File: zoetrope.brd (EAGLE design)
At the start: 68.6 x 53.3 mm, 9 parts

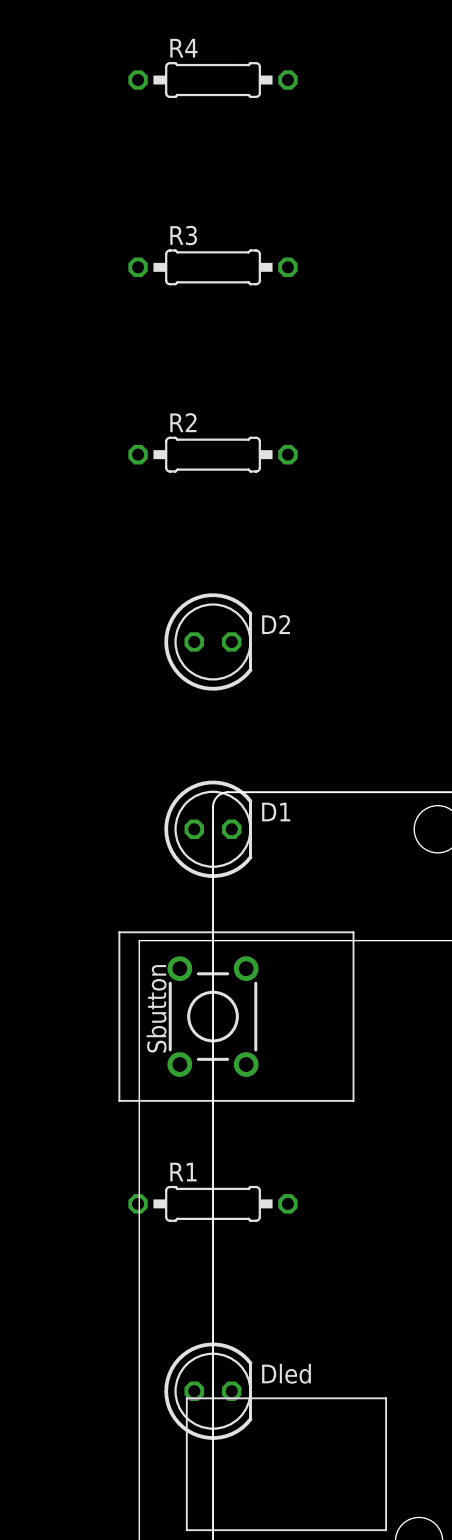
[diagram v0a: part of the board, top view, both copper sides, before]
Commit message: Added code and brd
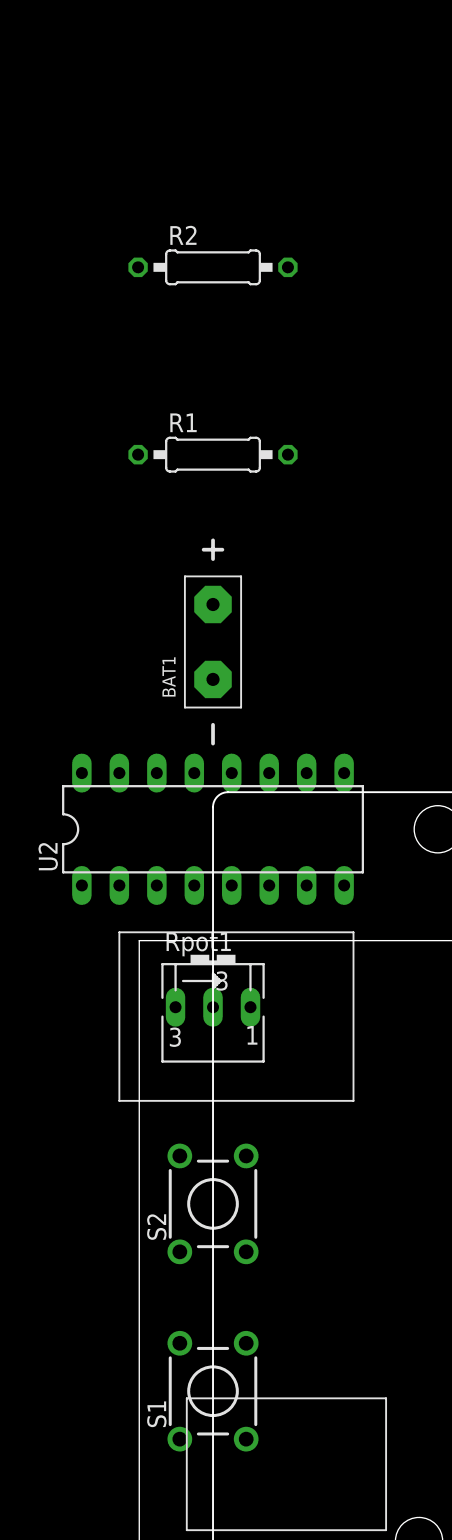
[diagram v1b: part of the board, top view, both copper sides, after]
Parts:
- removed D1, D2, Dled: (no value), AUTODESK_CIRCUITS_BREADBOARD:LED5MM
- removed R3, R4: 1k‎Ω, AUTODESK_CIRCUITS_BREADBOARD:0207/10
- removed Sbutton: (no value), AUTODESK_CIRCUITS_BREADBOARD:TL1105
- added BAT1: (no value), AUTODESK_CIRCUITS_BREADBOARD:DC-POWER
- added Rpot1: 250k‎Ω, AUTODESK_CIRCUITS_BREADBOARD:B25V
- added S1, S2: (no value), AUTODESK_CIRCUITS_BREADBOARD:TL1105
- added U2: (no value), AUTODESK_CIRCUITS_BREADBOARD:DIL16
- R1, R2: value 1k‎Ω -> 10000‎Ω
- moved R1 50.8 mm to (5.00, 86.3)
- moved R2 12.7 mm to (5.00, 99.0)
- renumbered Uboard to U1
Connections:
- new net N$12: U2.6
- new net N$13: U1.2, U2.7
- new net N$14: BAT1.+, U2.8
- new net N$15: U2.9
- new net N$16: U2.10
- new net N$17: U2.11
- new net N$18: U2.12
- new net N$19: U2.13
- new net N$20: U2.14
- new net N$21: U2.15
- new net N$22: Rpot1.A, S1.3, S2.3, U1.5V, U2.16
- net N$1: now also S1.4, U1.5; no longer R1.1, R2.1, R3.1, R4.1, U1.GND..
- net N$10: now also U2.3; no longer Sbutton.2
- net N$11: now also BAT1.-, R1.1, R2.1, Rpot1.E, U1.GND.., U2.4, U2.5; no longer Sbutton.1
- net N$2: now also R1.2, S1.2; no longer Sbutton.3, U1.5V
- net N$3: now also S1.1; no longer Dled.K, R4.2
- net N$4: now also S2.4, U1.4; no longer Dled.A, U1.3
- net N$5: now also R2.2, S2.2; no longer D2.K, R1.2
- net N$6: now also S2.1; no longer D2.A, U1.5
- net N$7: now also Rpot1.S; no longer D1.K, R3.2
- net N$8: now also U1.9, U2.1; no longer D1.A, U1.4
- net N$9: now also U1.3, U2.2; no longer R2.2, Sbutton.4, U1.2
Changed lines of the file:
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@@
 </autorouter>
 <elements>
-<element value="" name="Uboard" library="AUTODESK_CIRCUITS_BREADBOARD" package="ARDUINO_UNO" x="5" y="10.08"></element><element value="" name="Dled" library="AUTODESK_CIRCUITS_BREADBOARD" package="LED5MM" x="5" y="22.78"></element><element value="1k‎Ω" name="R1" library="AUTODESK_CIRCUITS_BREADBOARD" package="0207/10" x="5" y="35.480000000000004"></element><element value="" name="Sbutton" library="AUTODESK_CIRCUITS_BREADBOARD" package="TL1105" x="5" y="48.18"></element><element value="" name="D1" library="AUTODESK_CIRCUITS_BREADBOARD" package="LED5MM" x="5" y="60.879999999999995"></element><element value="" name="D2" library="AUTODESK_CIRCUITS_BREADBOARD" package="LED5MM" x="5" y="73.58"></element><element value="1k‎Ω" name="R2" library="AUTODESK_CIRCUITS_BREADBOARD" package="0207/10" x="5" y="86.28"></element><element value="1k‎Ω" name="R3" library="AUTODESK_CIRCUITS_BREADBOARD" package="0207/10" x="5" y="98.98"></element><element value="1k‎Ω" name="R4" library="AUTODESK_CIRCUITS_BREADBOARD" package="0207/10" x="5" y="111.68"></element></elements>
+<element value="" name="U1" library="AUTODESK_CIRCUITS_BREADBOARD" package="ARDUINO_UNO" x="5" y="10.08"></element><element value="" name="S1" library="AUTODESK_CIRCUITS_BREADBOARD" package="TL1105" x="5" y="22.78"></element><element value="" name="S2" library="AUTODESK_CIRCUITS_BREADBOARD" package="TL1105" x="5" y="35.480000000000004"></element><element value="250k‎Ω" name="Rpot1" library="AUTODESK_CIRCUITS_BREADBOARD" package="B25V" x="5" y="48.18"></element><element value="" name="U2" library="AUTODESK_CIRCUITS_BREADBOARD" package="DIL16" x="5" y="60.879999999999995"></element><element value="" name="BAT1" library="AUTODESK_CIRCUITS_BREADBOARD" package="DC-POWER" x="5" y="73.58"></element><element value="10000‎Ω" name="R1" library="AUTODESK_CIRCUITS_BREADBOARD" package="0207/10" x="5" y="86.28"></element><element value="10000‎Ω" name="R2" library="AUTODESK_CIRCUITS_BREADBOARD" package="0207/10" x="5" y="98.98"></element></elements>
 <signals>
-<signal name="N$1"><contactref element="Uboard" pad="GND.."></contactref><contactref element="R2" pad="1"></contactref><wire x1="45.64" y1="12.620000000000001" x2="-0.08000000000000007" y2="86.28" width="0" layer="19" extent="1-1"></wire><contactref element="R1" pad="1"></contactref><wire x1="-0.08000000000000007" y1="86.28" x2="-0.08000000000000007" y2="35.480000000000004" width="0" layer="19" extent="1-1"></wire><contactref element="R3" pad="1"></contactref><wire x1="-0.08000000000000007" y1="35.480000000000004" x2="-0.08000000000000007" y2="98.98" width="0" layer="19" extent="1-1"></wire><contactref element="R4" pad="1"></contactref><wire x1="-0.08000000000000007" y1="98.98" x2="-0.08000000000000007" y2="111.68" width="0" layer="19" extent="1-1"></wire></signal><signal name="N$2"><contactref element="Uboard" pad="5V"></contactref><contactref element="Sbutton" pad="3"></contactref><wire x1="43.1" y1="12.620000000000001" x2="2.75" y2="44.93" width="0" layer="19" extent="1-1"></wire></signal><signal name="N$3"><contactref element="Dled" pad="K"></contactref><contactref element="R4" pad="2"></contactref><wire x1="6.27" y1="22.78" x2="10.08" y2="111.68" width="0" layer="19" extent="1-1"></wire></signal><signal name="N$4"><contactref element="Dled" pad="A"></contactref><contactref element="Uboard" pad="3"></contactref><wire x1="3.73" y1="22.78" x2="60.88" y2="60.879999999999995" width="0" layer="19" extent="1-1"></wire></signal><signal name="N$5"><contactref element="D2" pad="K"></contactref><contactref element="R1" pad="2"></contactref><wire x1="6.27" y1="73.58" x2="10.08" y2="35.480000000000004" width="0" layer="19" extent="1-1"></wire></signal><signal name="N$6"><contactref element="D2" pad="A"></contactref><contactref element="Uboard" pad="5"></contactref><wire x1="3.73" y1="73.58" x2="55.8" y2="60.879999999999995" width="0" layer="19" extent="1-1"></wire></signal><signal name="N$7"><contactref element="D1" pad="K"></contactref><contactref element="R3" pad="2"></contactref><wire x1="6.27" y1="60.879999999999995" x2="10.08" y2="98.98" width="0" layer="19" extent="1-1"></wire></signal><signal name="N$8"><contactref element="D1" pad="A"></contactref><contactref element="Uboard" pad="4"></contactref><wire x1="3.73" y1="60.879999999999995" x2="58.34" y2="60.879999999999995" width="0" layer="19" extent="1-1"></wire></signal><signal name="N$9"><contactref element="Sbutton" pad="4"></contactref><contactref element="Uboard" pad="2"></contactref><wire x1="7.25" y1="44.93" x2="63.42" y2="60.879999999999995" width="0" layer="19" extent="1-1"></wire><contactref element="R2" pad="2"></contactref><wire x1="63.42" y1="60.879999999999995" x2="10.08" y2="86.28" width="0" layer="19" extent="1-1"></wire></signal><signal name="N$10"><contactref element="Sbutton" pad="2"></contactref></signal><signal name="N$11"><contactref element="Sbutton" pad="1"></contactref></signal></signals>
+<signal name="N$1"><contactref element="S1" pad="4"></contactref><contactref element="U1" pad="5"></contactref><wire x1="7.25" y1="19.53" x2="55.8" y2="60.879999999999995" width="0" layer="19" extent="1-1"></wire></signal><signal name="N$2"><contactref element="S1" pad="2"></contactref><contactref element="R1" pad="2"></contactref><wire x1="7.25" y1="26.03" x2="10.08" y2="86.28" width="0" layer="19" extent="1-1"></wire></signal><signal name="N$3"><contactref element="S1" pad="1"></contactref></signal><signal name="N$4"><contactref element="S2" pad="4"></contactref><contactref element="U1" pad="4"></contactref><wire x1="7.25" y1="32.230000000000004" x2="58.34" y2="60.879999999999995" width="0" layer="19" extent="1-1"></wire></signal><signal name="N$5"><contactref element="S2" pad="2"></contactref><contactref element="R2" pad="2"></contactref><wire x1="7.25" y1="38.730000000000004" x2="10.08" y2="98.98" width="0" layer="19" extent="1-1"></wire></signal><signal name="N$6"><contactref element="S2" pad="1"></contactref></signal><signal name="N$7"><contactref element="Rpot1" pad="S"></contactref></signal><signal name="N$8"><contactref element="U2" pad="1"></contactref><contactref element="U1" pad="9"></contactref><wire x1="-3.8900000000000006" y1="57.06999999999999" x2="44.116" y2="60.879999999999995" width="0" layer="19" extent="1-1"></wire></signal><signal name="N$9"><contactref element="U2" pad="2"></contactref><contactref element="U1" pad="3"></contactref><wire x1="-1.3499999999999996" y1="57.06999999999999" x2="60.88" y2="60.879999999999995" width="0" layer="19" extent="1-1"></wire></signal><signal name="N$10"><contactref element="U2" pad="3"></contactref></signal><signal name="N$11"><contactref element="U2" pad="5"></contactref><contactref element="U2" pad="4"></contactref><wire x1="6.27" y1="57.06999999999999" x2="3.73" y2="57.06999999999999" width="0" layer="19" extent="1-1"></wire><contactref element="Rpot1" pad="E"></contactref><wire x1="3.73" y1="57.06999999999999" x2="2.46" y2="48.815" width="0" layer="19" extent="1-1"></wire><contactref element="U1" pad="GND.."></contactref><wire x1="2.46" y1="48.815" x2="45.64" y2="12.620000000000001" width="0" layer="19" extent="1-1"></wire><contactref element="BAT1" pad="-"></contactref><wire x1="45.64" y1="12.620000000000001" x2="5" y2="71.03999999999999" width="0" layer="19" extent="1-1"></wire><contactref element="R1" pad="1"></contactref><wire x1="5" y1="71.03999999999999" x2="-0.08000000000000007" y2="86.28" width="0" layer="19" extent="1-1"></wire><contactref element="R2" pad="1"></contactref><wire x1="-0.08000000000000007" y1="86.28" x2="-0.08000000000000007" y2="98.98" width="0" layer="19" extent="1-1"></wire></signal><signal name="N$12"><contactref element="U2" pad="6"></contactref></signal><signal name="N$13"><contactref element="U2" pad="7"></contactref><contactref element="U1" pad="2"></contactref><wire x1="11.35" y1="57.06999999999999" x2="63.42" y2="60.879999999999995" width="0" layer="19" extent="1-1"></wire></signal><signal name="N$14"><contactref element="U2" pad="8"></contactref><contactref element="BAT1" pad="+"></contactref><wire x1="13.89" y1="57.06999999999999" x2="5" y2="76.12" width="0" layer="19" extent="1-1"></wire></signal><signal name="N$15"><contactref element="U2" pad="9"></contactref></signal><signal name="N$16"><contactref element="U2" pad="10"></contactref></signal><signal name="N$17"><contactref element="U2" pad="11"></contactref></signal><signal name="N$18"><contactref element="U2" pad="12"></contactref></signal><signal name="N$19"><contactref element="U2" pad="13"></contactref></signal><signal name="N$20"><contactref element="U2" pad="14"></contactref></signal><signal name="N$21"><contactref element="U2" pad="15"></contactref></signal><signal name="N$22"><contactref element="U2" pad="16"></contactref><contactref element="Rpot1" pad="A"></contactref><wire x1="-3.8900000000000006" y1="64.69" x2="7.54" y2="48.815" width="0" layer="19" extent="1-1"></wire><contactref element="S2" pad="3"></contactref><wire x1="7.54" y1="48.815" x2="2.75" y2="32.230000000000004" width="0" layer="19" extent="1-1"></wire><contactref element="S1" pad="3"></contactref><wire x1="2.75" y1="32.230000000000004" x2="2.75" y2="19.53" width="0" layer="19" extent="1-1"></wire><contactref element="U1" pad="5V"></contactref><wire x1="2.75" y1="19.53" x2="43.1" y2="12.620000000000001" width="0" layer="19" extent="1-1"></wire></signal></signals>
 </board>
 </drawing>
